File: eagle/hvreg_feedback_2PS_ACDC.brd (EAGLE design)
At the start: 137.9 x 101.6 mm, 18 parts

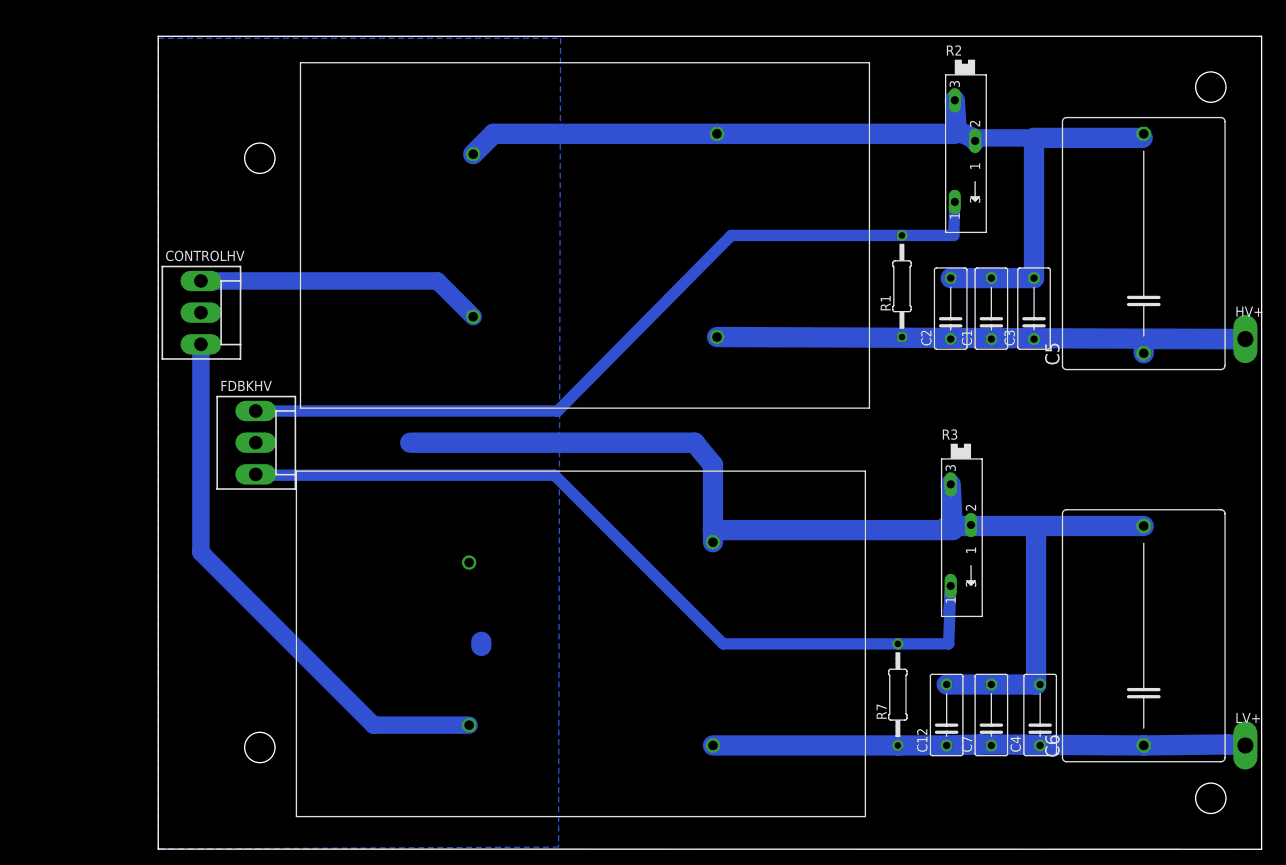
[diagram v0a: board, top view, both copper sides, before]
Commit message: IXYS board solution, gatedriver components
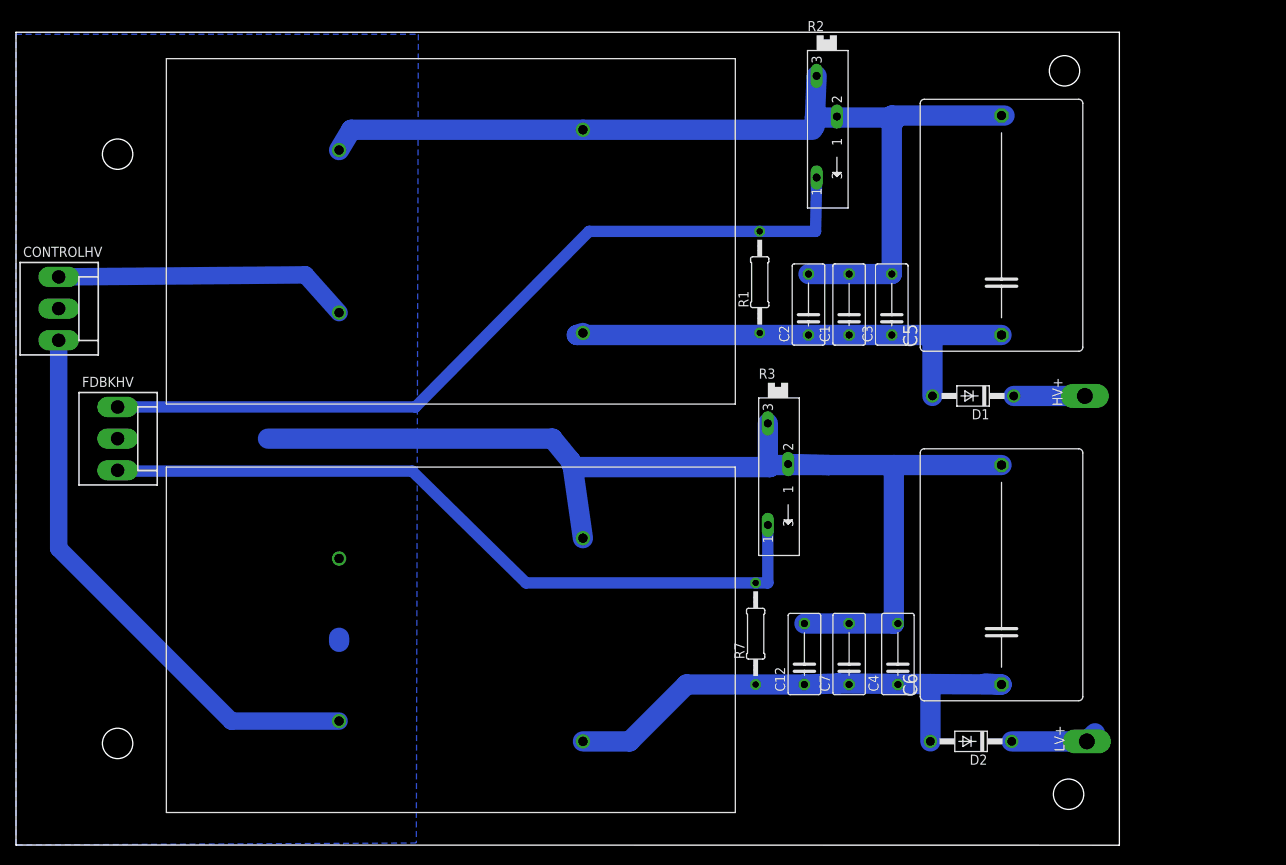
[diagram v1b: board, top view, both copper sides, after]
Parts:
- added D1, D2: 1N4004, diode:DO41-10
- moved R3 24.1 mm to (95.2, 46.0)
- moved HV+ 21.3 mm to (133.6, 56.4), turned to 90 degrees
- moved LV+ 19.8 mm to (133.9, 13.2), turned to 90 degrees
- moved C6 19.3 mm to (123.2, 34.0)
- moved C7 19.3 mm to (104.1, 24.1)
- moved R7 19.3 mm to (92.5, 26.7)
- moved C12 19.3 mm to (98.6, 24.1)
- moved C4 19.3 mm to (110.2, 24.1)
- moved C5 17.9 mm to (123.2, 77.7)
- moved C1 17.8 mm to (104.1, 67.8)
- moved C2 17.8 mm to (99.1, 67.8)
- moved C3 17.8 mm to (109.5, 67.8)
- moved CONTROLHV 17.8 mm to (5.33, 67.3)
- moved R1 17.8 mm to (93.0, 70.6)
- moved R2 17.5 mm to (101.3, 89.4)
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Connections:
- new net N$6: D1.C, HV+.TP
- new net N$7: D2.C, LV+.TP
- net N$1: now also D1.A; no longer HV+.TP
- net N$2: now also D2.A; no longer LV+.TP
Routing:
- net N$1: track 80.5 -> 61.0 mm
- net N$8: track 106.3 -> 95.1 mm
- net N$7: track 0.00 -> 10.8 mm
- net N$6: track 0.00 -> 10.2 mm
- net GND: track 258.4 -> 267.2 mm
- net N$3: track 100.6 -> 103.1 mm
- net N$2: track 66.6 -> 64.5 mm
- net N$5: track 68.5 -> 70.0 mm
- net N$4: track 35.9 -> 37.2 mm
